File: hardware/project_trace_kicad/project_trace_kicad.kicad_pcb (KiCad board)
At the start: 4 copper layers, 100 x 100 mm, 111 parts, among them J204 Screw_Terminal_01x04, J205 Conn_Coaxial, J503 Screw_Terminal_01x04, J602 Conn_01x14_Socket, U201 TLE2426xLP, U202 AQW280SX, U203 AQW282SX, U204 OPA2837IRUNT, U205 TS5A23159DGS, U206 OPA2837IRUNT, U207 SN74LVC2G14DBV, U301 THS4131IDR, U303 ADS1602, U304 MCP6499T, U306 LM4040DBZ-4.1, U501 UA78M33QDCYRQ1, U502 UA78M05QDCYRQ1, U503 NUCLEO-H753ZI

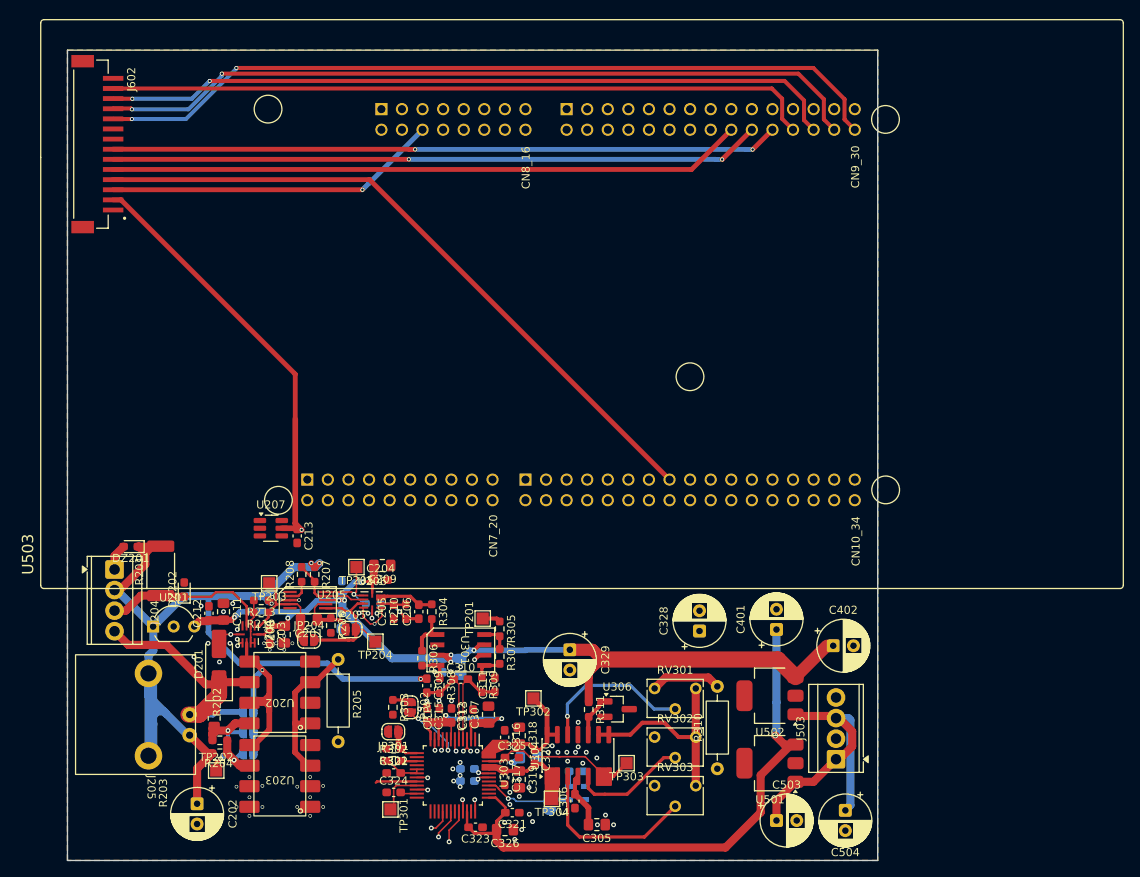
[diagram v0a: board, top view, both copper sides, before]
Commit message: Work on Layout
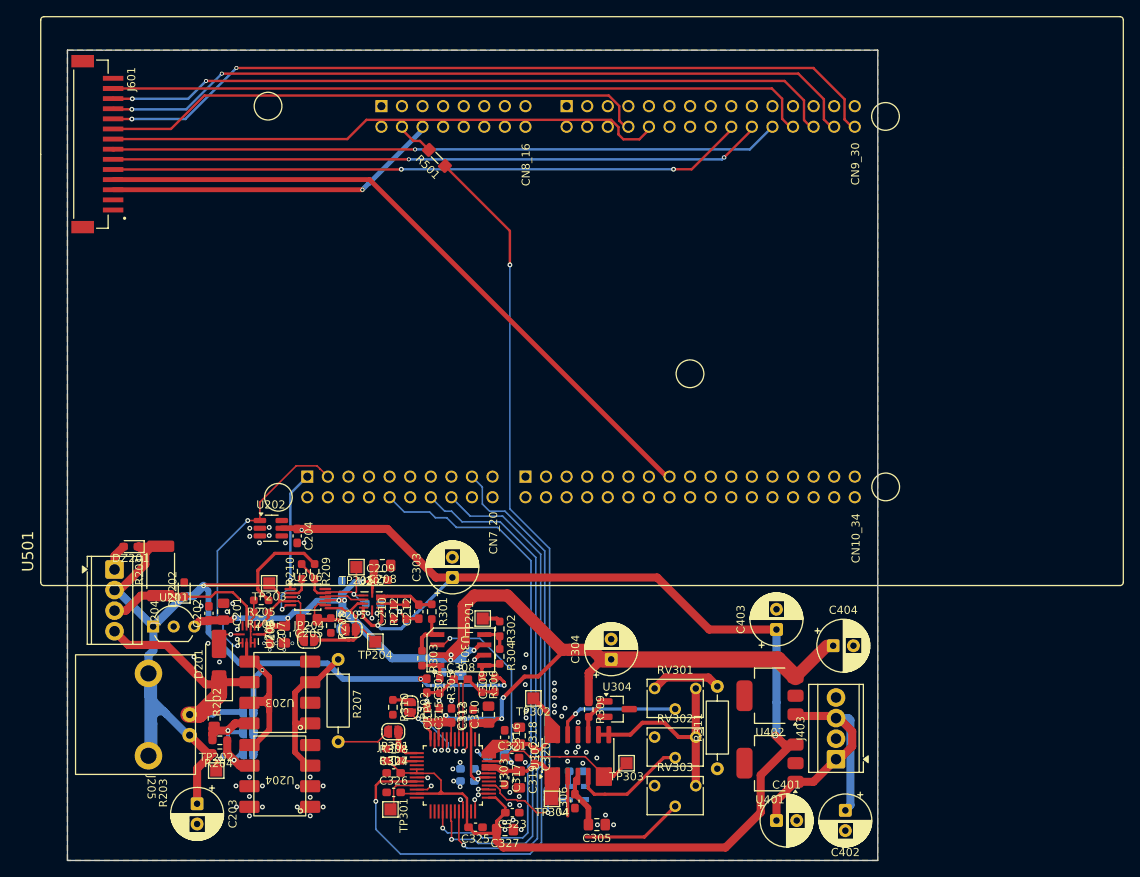
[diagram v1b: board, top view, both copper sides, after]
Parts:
- added R501: 100, ProjectTraceFootprints:RN73R2ATTD1000B25, F.Cu at (145.6, 63.3)
- U206: renamed from U205; footprint ProjectTraceFootprints:SOIC-10 - DGS0010A -> Package_SO:TSSOP-10_3x3mm_P0.5mm
- moved C303 31.2 mm to (147.5, 115.1)
- moved C304 5.24 mm to (167.1, 125.2), turned to 90 degrees
- moved C322 4.04 mm to (152.9, 137.0), turned to 180 degrees
- moved JP303 1.30 mm to (159.5, 141.9), turned to -90 degrees
- moved R209 0.37 mm to (130.5, 114.3)
- moved R210 0.37 mm to (128.9, 114.3)
- moved U206 0.37 mm to (129.7, 117.5), turned to 0 degrees
- moved U501 0.37 mm to (163.5, 81.0)
- renumbered C211 to C201, C212 to C202, C202 to C203, C213 to C204, C201 to C205, C208 to C206, C203 to C207, C209 to C208, C204 to C209, C205 to C210, C210 to C211, C206 to C212, C207 to C213, C328 to C303, C329 to C304, C309 to C307, C310 to C308, C311 to C309, C307 to C310, C308 to C311, C325 to C321, C327 to C322, C321 to C323, C322 to C324, C323 to C325, C324 to C326, C326 to C327, C304 to C328, C303 to C329, C503 to C401, C504 to C402, C401 to C403, C402 to C404, J503 to J403, J602 to J601, R213 to R205, R212 to R206, R205 to R207, R206 to R208, R207 to R209, R208 to R210, R209 to R211, R210 to R212, R304 to R301, R305 to R302, R306 to R303, R307 to R304, R308 to R305, R309 to R306, R301 to R307, R302 to R308, R311 to R309, R303 to R310, R310 to R311, U207 to U202, U202 to U203, U203 to U204, U204 to U205, U206 to U207, U304 to U302, U306 to U304, U302 to U305, U501 to U401, U502 to U402, U503 to U501
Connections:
- C324 pad 2: unconnected-(C322-Pad2) -> +3V3
- R309 pad 2: Net-(U304C-+) -> Net-(U302C-+)
- U302 pad 10: Net-(U304C-+) -> Net-(U302C-+)
- U304 pad 1: unconnected-(U306-K-Pad1) -> Net-(U302C-+)
- U501 pad 7_1: unconnected-(U503B-PC6-Pad7_1) -> /Inputs/20dBGain.EN
- U501 pad 7_11: unconnected-(U503B-PC7-Pad7_11) -> /Inputs/0dBAtten.~{EN}
- U501 pad 7_15: unconnected-(U503B-PB3-Pad7_15) -> /Inputs/ACCouple.~{EN}
- U501 pad 7_3: unconnected-(U503B-PB15-Pad7_3) -> /Inputs/VOLT/~{AMP}
- U501 pad 7_5: unconnected-(U503B-PB13-Pad7_5) -> /Inputs/-20dBAtten.~{EN}
- U501 pad 7_7: unconnected-(U503B-PB12-Pad7_7) -> /Inputs/-40dBAtten.~{EN}
- U501 pad 8_2: unconnected-(U503C-PC8-Pad8_2) -> /ADC/CLK.EN
- U501 pad 8_4: unconnected-(U503C-PC9-Pad8_4) -> Net-(U501C-PC9)
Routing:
- net /ADC/CLK.BAC: track 0.00 -> 82.3 mm, vias 0 -> 1
- net /ADC/SYNC: track 5.11 -> 83.1 mm, vias 0 -> 1
- net /Measurement and Analysis Module/SW2: track 0.00 -> 69.1 mm
- net /Measurement and Analysis Module/SW1: track 0.00 -> 68.1 mm
- net /ADC/SCLK: track 2.96 -> 67.7 mm
- net /ADC/DOUT: track 3.78 -> 64.7 mm
- net /ADC/FSO: track 4.25 -> 63.4 mm
- net /Inputs/VOLT/~{AMP}: track 0.75 -> 33.7 mm, vias 1 -> 2
- net +3V3: track 157.5 -> 188.5 mm
- net +5V: track 148.9 -> 176.7 mm, vias 11 -> 12
- net +2V5: track 22.2 -> 44.2 mm, vias 1 -> 2
- net VCOM: track 132.1 -> 146.9 mm, vias 5 -> 3
- net /Inputs/20dBGain.EN: track 0.00 -> 14.7 mm, vias 0 -> 1
- net /Inputs/ACCouple.~{EN}: track 0.00 -> 4.85 mm, vias 0 -> 1
- net Net-(U304C-+): track 4.46 -> 0.00 mm
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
